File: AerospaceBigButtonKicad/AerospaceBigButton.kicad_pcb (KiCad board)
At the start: 2 copper layers, 120 x 80 mm, 20 parts, among them J1 Conn_01x07, J2 Conn_01x07, J3 Conn_01x02, J4 Conn_01x02, J5 Conn_01x02, Q1 Si7336ADP, SW1 BIGSWITCH, U1 AMS1117-5.0

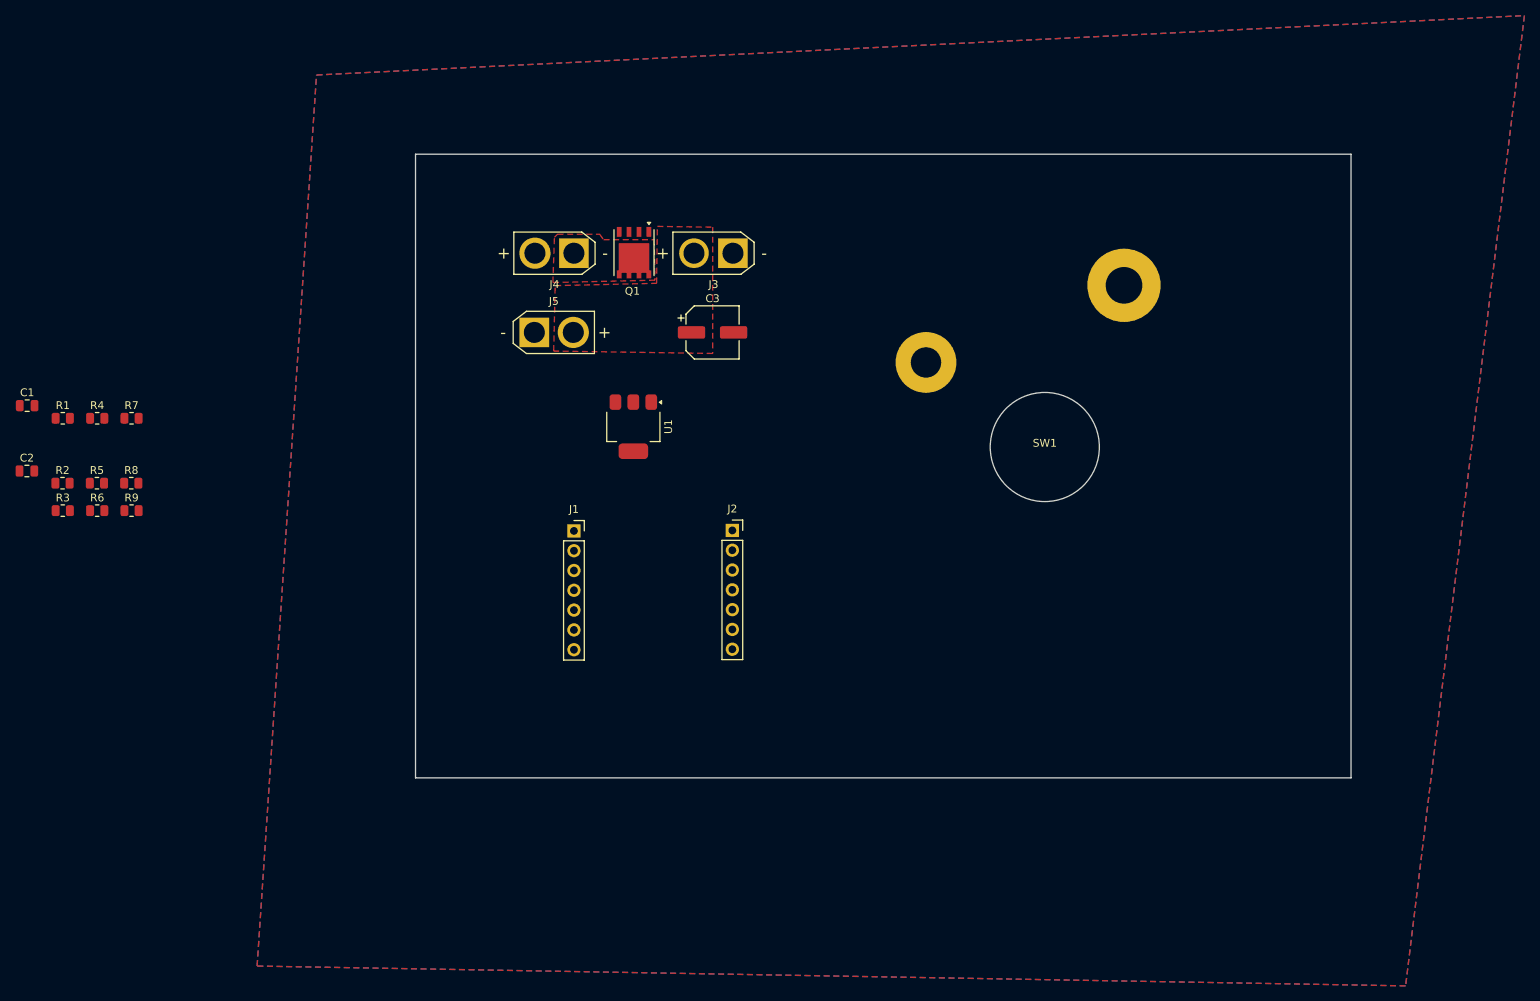
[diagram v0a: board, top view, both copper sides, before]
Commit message: basic design done
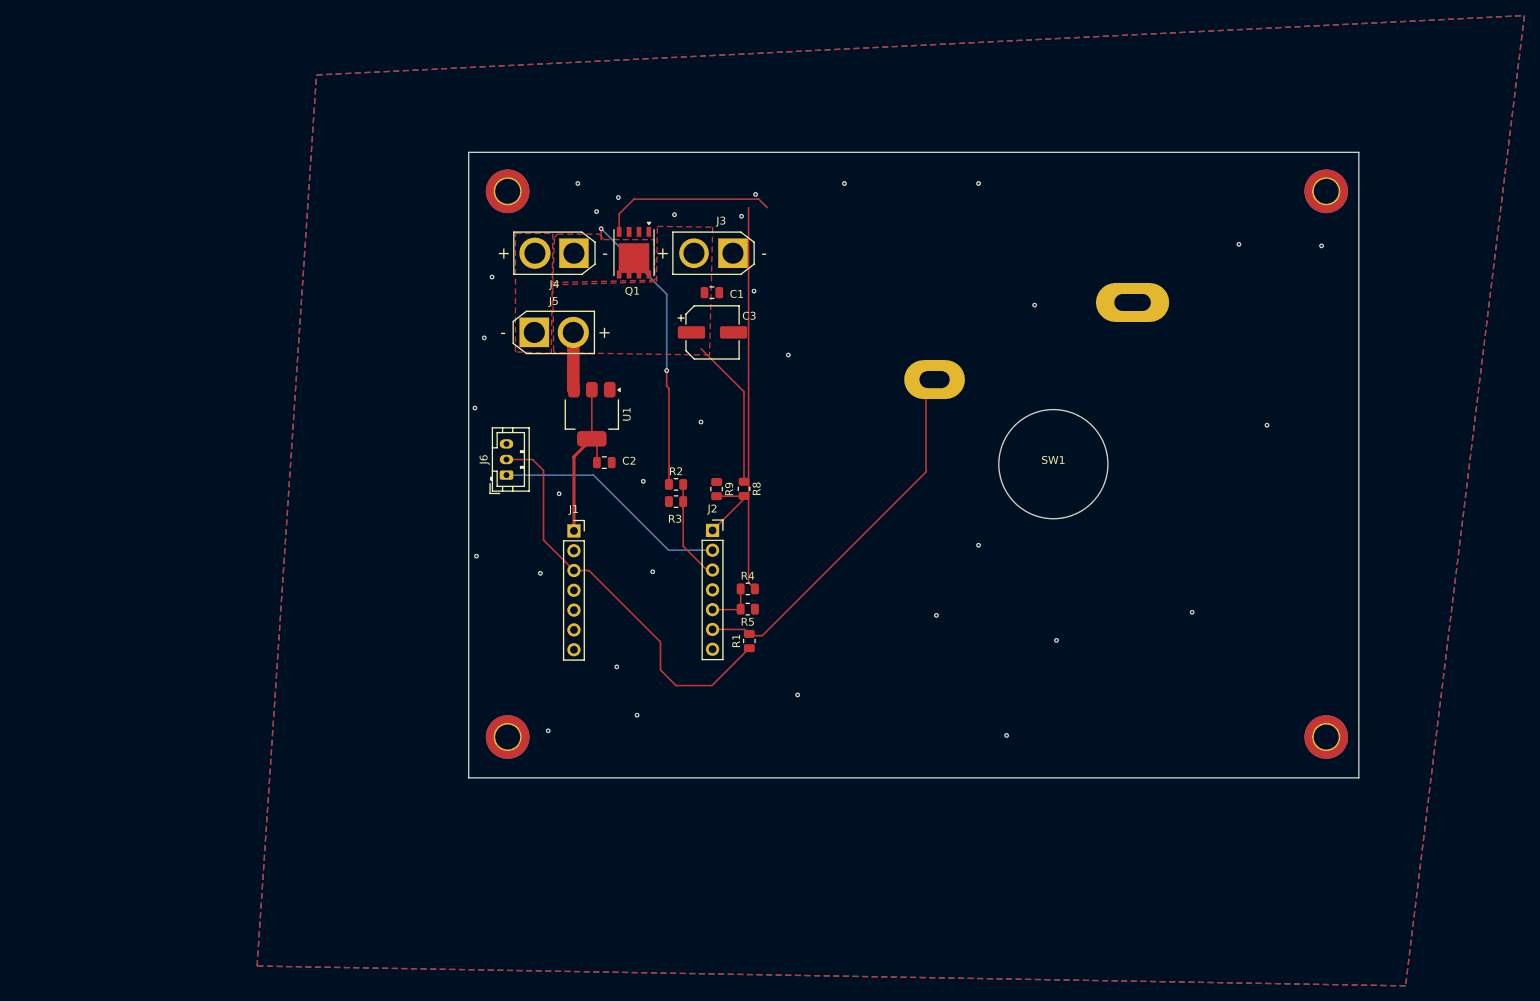
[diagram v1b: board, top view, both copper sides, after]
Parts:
- removed R6: 100k, Resistor_SMD:R_0805_2012Metric
- removed R7: 27k, Resistor_SMD:R_0805_2012Metric
- added H1: MountingHole_Pad, MountingHole:MountingHole_3.2mm_M3_DIN965_Pad_TopBottom, F.Cu at (55.0, 20.0)
- added H2: MountingHole_Pad, MountingHole:MountingHole_3.2mm_M3_DIN965_Pad_TopBottom, F.Cu at (160.0, 20.0)
- added H3: MountingHole_Pad, MountingHole:MountingHole_3.2mm_M3_DIN965_Pad_TopBottom, F.Cu at (160.0, 90.0)
- added H4: MountingHole_Pad, MountingHole:MountingHole_3.2mm_M3_DIN965_Pad_TopBottom, F.Cu at (55.0, 90.0)
- added J6: Conn_01x03, Connector_JST:JST_PH_B3B-PH-K_1x03_P2.00mm_Vertical, F.Cu at (54.9, 56.4)
- moved R1 92.6 mm to (86.0, 77.7), turned to 90 degrees
- moved C1 89.0 mm to (81.2, 33.0)
- moved R4 86.3 mm to (85.8, 71.0)
- moved R5 85.0 mm to (85.8, 73.6), turned to 180 degrees
- moved R2 78.7 mm to (76.6, 57.6)
- moved R3 78.7 mm to (76.6, 59.8)
- moved R8 78.6 mm to (85.3, 58.2), turned to -90 degrees
- moved R9 75.1 mm to (81.8, 58.2), turned to -90 degrees
- moved C2 74.1 mm to (67.4, 54.8)
- moved U1 5.55 mm to (65.8, 48.6)
- moved J2 2.54 mm to (81.3, 63.5)
- moved SW1 2.46 mm to (125.0, 55.0)
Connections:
- J2 pad 3: /RGB -> /CONT
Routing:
- net Net-(Q1-G): track 0.00 -> 71.8 mm
- net +3V3: track 0.00 -> 52.5 mm
- net /BIGSWITCH: track 0.00 -> 50.5 mm
- net Net-(J4-Pin_1): track 0.00 -> 37.8 mm, vias 0 -> 2
- net /ARMED: track 0.00 -> 30.4 mm
- net VCC: track 0.00 -> 26.7 mm
- net +5V: track 0.00 -> 22.4 mm
- net /CONT: track 0.00 -> 13.1 mm
- net /VINSENSE: track 0.00 -> 9.63 mm
- net /FIRE: track 0.00 -> 6.23 mm
- net GND: vias 0 -> 32
- added copper zone on F.Cu, net /PYRO
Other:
- board size 120 x 80 mm -> 114.2 x 80.2 mm
